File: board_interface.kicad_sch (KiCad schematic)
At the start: 70 parts, among them J81 Conn_01x02, SW81 SW_SPDT, SW82 SW_SPDT, SW83 SW_SPDT, SW84 SW_SPDT, SW85 SW_SPDT, SW86 SW_SPDT, SW87 SW_SPDT, SW88 SW_SPDT, SW89 SW_SPDT, SW90 SW_SPDT, SW91 SW_SPDT, SW92 SW_SPDT, SW93 SW_SPDT, SW94 SW_SPDT, SW95 SW_SPDT, SW96 SW_SPDT, SW97 SW_SPDT

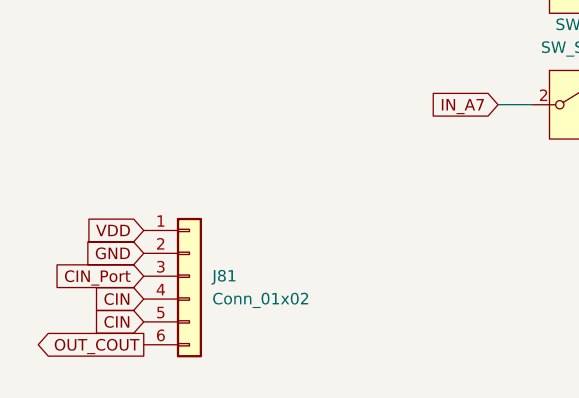
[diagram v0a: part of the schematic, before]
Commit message: FA 1-bit PCB Ok
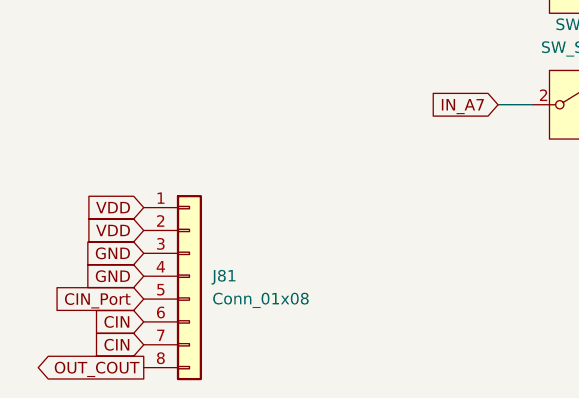
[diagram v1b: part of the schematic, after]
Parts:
- J81: value Conn_01x02 -> Conn_01x08; footprint Connector_PinHeader_2.54mm:PinHeader_1x02_P2.54mm_Horizontal -> Connector_PinHeader_2.54mm:PinHeader_1x08_P2.54mm_Horizontal; symbol Connector_Generic:Conn_01x06 -> Connector_Generic:Conn_01x08
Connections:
- net CIN: now also J81.6 (Pin_6), J81.7 (Pin_7); no longer J81.4 (Pin_4), J81.5 (Pin_5)
- net CIN_Port: now also J81.5 (Pin_5); no longer J81.3 (Pin_3)
- net GND: now also J81.3 (Pin_3), J81.4 (Pin_4); no longer J81.2 (Pin_2)
- net OUT_COUT: now also J81.8 (Pin_8); no longer J81.6 (Pin_6)
- net VDD: now also J81.2 (Pin_2)
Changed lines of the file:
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@@
 	(global_label "CIN_Port"
 		(shape input)
-		(at 27.94 140.97 180)
+		(at 27.94 143.51 180)
 		(fields_autoplaced yes)
 		(effects
@@
 		)
 		(property "Intersheetrefs" "${INTERSHEET_REFS}"
-			(at 16.851 140.97 0)
+			(at 16.851 143.51 0)
 			(effects
 				(font
@@
 	(global_label "CIN"
 		(shape input)
-		(at 27.94 143.51 180)
+		(at 27.94 146.05 180)
 		(fields_autoplaced yes)
 		(effects
@@
 		)
 		(property "Intersheetrefs" "${INTERSHEET_REFS}"
-			(at 21.7495 143.51 0)
+			(at 21.7495 146.05 0)
 			(effects
 				(font
@@
 	(global_label "OUT_COUT"
 		(shape output)
-		(at 27.94 148.59 180)
+		(at 27.94 151.13 180)
 		(fields_autoplaced yes)
 		(effects
@@
 		)
 		(property "Intersheetrefs" "${INTERSHEET_REFS}"
-			(at 15.46 148.59 0)
+			(at 15.46 151.13 0)
 			(effects
 				(font
@@
 	(global_label "CIN"
 		(shape input)
-		(at 27.94 146.05 180)
+		(at 27.94 148.59 180)
 		(fields_autoplaced yes)
 		(effects
@@
 		)
 		(property "Intersheetrefs" "${INTERSHEET_REFS}"
-			(at 21.7495 146.05 0)
+			(at 21.7495 148.59 0)
 			(effects
 				(font
@@
 		)
 	)
+	(global_label "GND"
+		(shape input)
+		(at 27.94 140.97 180)
+		(fields_autoplaced yes)
+		(effects
+			(font
+				(size 1.27 1.27)
+			)
+			(justify right)
+		)
+		(property "Intersheetrefs" "${INTERSHEET_REFS}"
+			(at 21.0843 140.97 0)
+			(effects
+				(font
+					(size 1.27 1.27)
+				)
+				(justify right)
+				(hide yes)
+			)
+		)
+	)
 	(global_label "VDD"
 		(shape input)
@@
 	(global_label "VDD"
 		(shape input)
-		(at 27.94 135.89 180)
+		(at 27.94 133.35 180)
 		(fields_autoplaced yes)
 		(effects
@@
 		)
 		(property "Intersheetrefs" "${INTERSHEET_REFS}"
-			(at 21.3262 135.89 0)
+			(at 21.3262 133.35 0)
 			(effects
 				(font
@@
 		)
 	)
+	(global_label "VDD"
+		(shape input)
+		(at 27.94 135.89 180)
+		(fields_autoplaced yes)
+		(effects
+			(font
+				(size 1.27 1.27)
+			)
+			(justify right)
+		)
+		(property "Intersheetrefs" "${INTERSHEET_REFS}"
+			(at 21.3262 135.89 0)
+			(effects
+				(font
+					(size 1.27 1.27)
+				)
+				(justify right)
+				(hide yes)
+			)
+		)
+	)
 	(global_label "GND"
 		(shape input)
@@
 	)
 	(symbol
-		(lib_id "Connector_Generic:Conn_01x06")
+		(lib_id "Connector_Generic:Conn_01x08")
 		(at 33.02 140.97 0)
 		(unit 1)
@@
 			)
 		)
-		(property "Value" "Conn_01x02"
+		(property "Value" "Conn_01x08"
 			(at 35.56 143.5099 0)
 			(effects
@@
 			)
 		)
-		(property "Footprint" "Connector_PinHeader_2.54mm:PinHeader_1x02_P2.54mm_Horizontal"
+		(property "Footprint" "Connector_PinHeader_2.54mm:PinHeader_1x08_P2.54mm_Horizontal"
 			(at 33.02 140.97 0)
 			(effects
@@
 			)
 		)
-		(property "Description" "Generic connector, single row, 01x06, script generated (kicad-library-utils/schlib/autogen/connector/)"
+		(property "Description" "Generic connector, single row, 01x08, script generated (kicad-library-utils/schlib/autogen/connector/)"
 			(at 33.02 140.97 0)
 			(effects
@@
 		(pin "6"
 		)
+		(pin "7"
+		)
+		(pin "8"
+		)
 		(instances

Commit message: BOM and Picture
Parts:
- D100, D101, D102, D103, D104, D105, D106, D81, D82, D83, D87, D88, D89, D90, D91, D92, D93, D94, D95, D96, D97, D98, D99: Equipment Link (none) -> https://nshopvn.com/product/led-duc-5mm-xanh-la-xanh-duong-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
- J81: Equipment Link (none) -> https://www.thegioiic.com/hang-rao-duc-don-2-54mm-40-chan-c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
- R137, R138, R139, R143, R144, R145, R146, R147, R148, R149, R150, R151, R152, R153, R154, R155, R156, R157, R158, R159, R160, R161, R162: Equipment Link (none) -> https://www.thegioiic.com/dien-tro-47-kohm-1-2w-5-4-vong-mau
- SW81, SW82, SW85, SW86, SW87, SW88, SW89, SW90, SW91, SW92, SW93, SW94, SW95, SW96, SW97: Equipment Link (none) -> https://www.thegioiic.com/ss-12d07vg4-cong-tac-truot-5-chan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
